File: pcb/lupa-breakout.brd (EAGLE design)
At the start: 40.3 x 40.6 mm, 16 parts

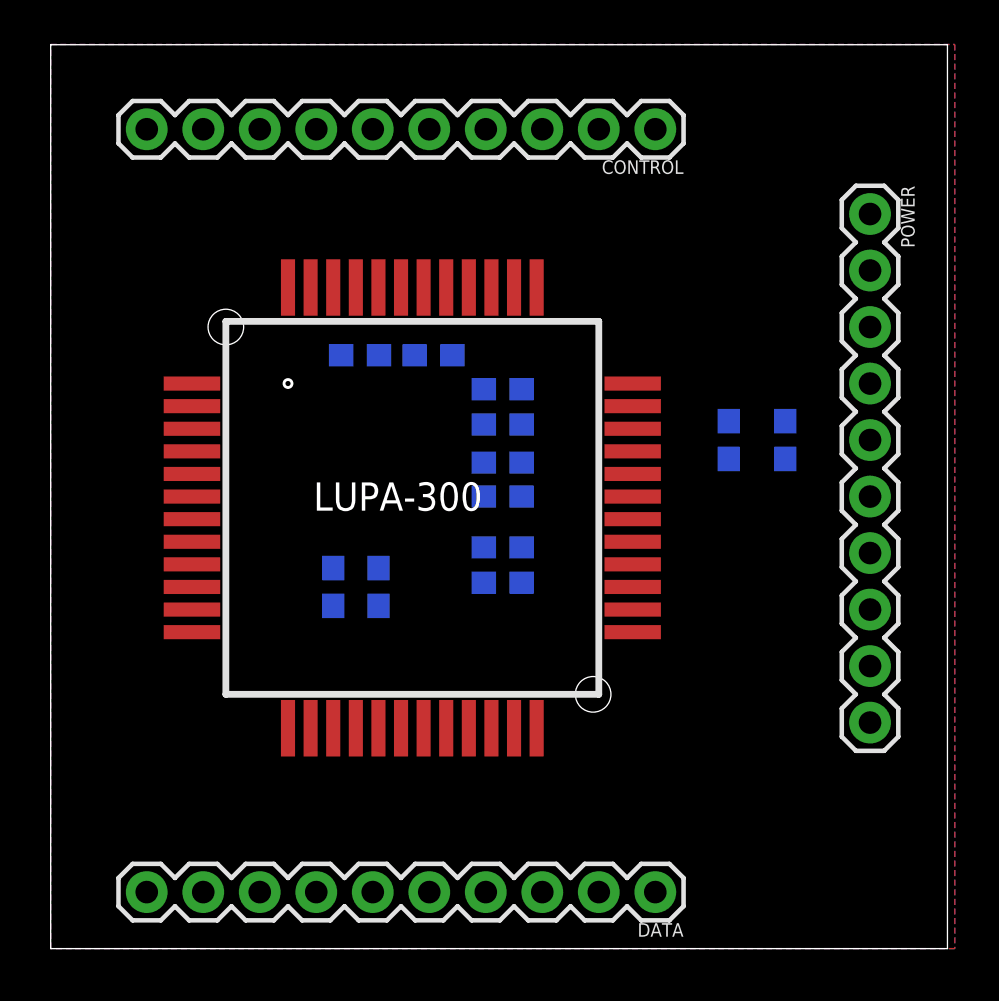
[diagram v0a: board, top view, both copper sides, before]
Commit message: more work on breakout
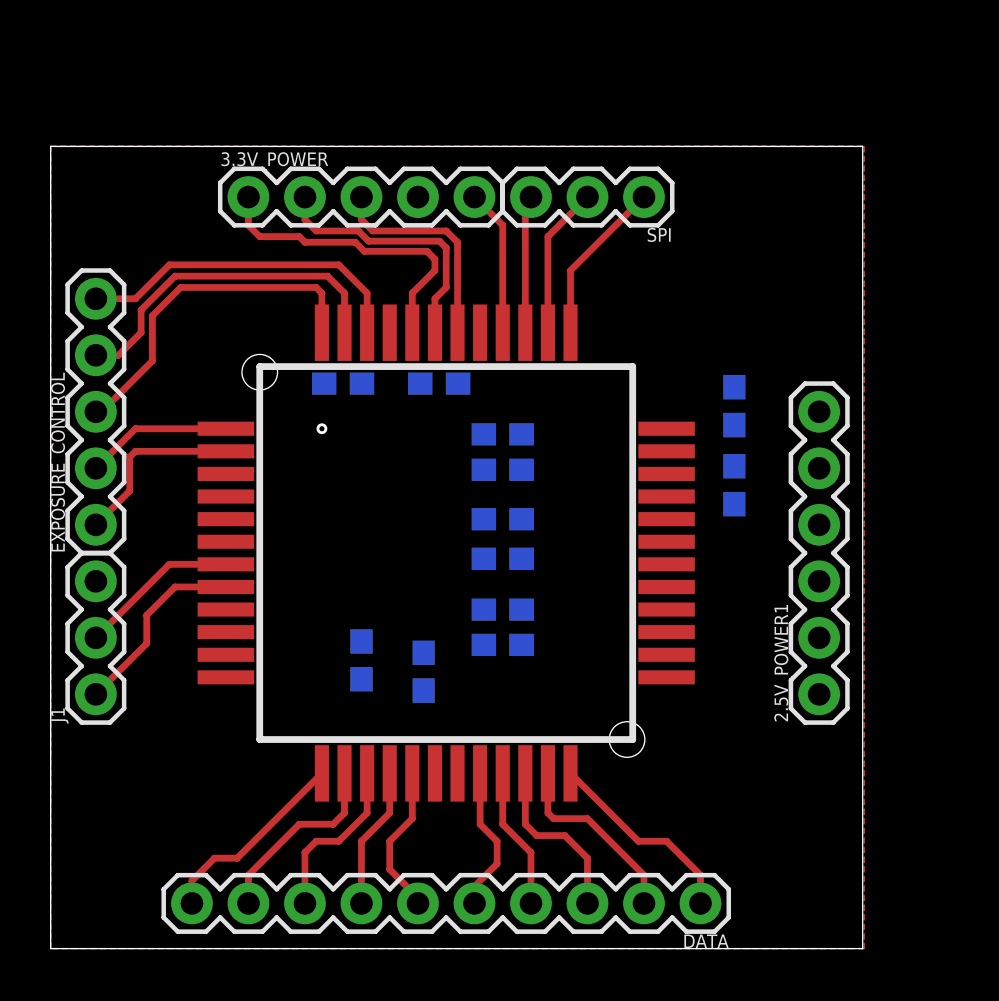
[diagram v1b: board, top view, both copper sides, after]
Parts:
- removed CONTROL, POWER: (no value), SparkFun-Connectors:1X10
- added 2.5V_POWER1: (no value), SparkFun-Connectors:1X06
- added 3.3V_POWER, EXPOSURE_CONTROL: (no value), SparkFun-Connectors:1X05
- added J1, SPI: 455-1750-1-ND, SparkFun-Connectors:1X03
- moved C1 4.32 mm to (16.8, 12.4), turned to 270 degrees
- moved R1 3.54 mm to (14.0, 13.0), turned to 270 degrees
- moved C4 2.79 mm to (20.3, 13.7)
- moved R3 2.79 mm to (20.3, 17.5)
- moved R4 2.79 mm to (20.3, 15.2)
- moved C2 2.75 mm to (30.7, 24.4), turned to 90 degrees
- moved C3 2.54 mm to (20.3, 19.3)
- moved U$1 2.54 mm to (10.7, 10.7)
- moved DATA 2.09 mm to (29.2, 2.03)
- moved R2 2.05 mm to (30.7, 20.8)
- moved C5 2.03 mm to (20.3, 23.1)
- moved R5 2.03 mm to (20.3, 21.5)
- moved C6 1.48 mm to (13.1, 25.4)
- moved R6 1.30 mm to (17.5, 25.4)
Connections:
- net CLK: now also J1.1; no longer CONTROL.10
- net FRAME_VALID: now also EXPOSURE_CONTROL.4; no longer CONTROL.5
- net GND: now also 2.5V_POWER1.1, 3.3V_POWER.4, J1.3; no longer POWER.10
- net INT_TIME1: now also EXPOSURE_CONTROL.1; no longer CONTROL.8
- net INT_TIME2: now also EXPOSURE_CONTROL.2; no longer CONTROL.7
- net INT_TIME3: now also EXPOSURE_CONTROL.3; no longer CONTROL.6
- net LINE_VALID: now also EXPOSURE_CONTROL.5; no longer CONTROL.4
- net RESET: now also J1.2; no longer CONTROL.9
- net SPI_CLK: now also SPI.2; no longer CONTROL.2
- net SPI_DATA: now also SPI.3; no longer CONTROL.3
- net SPI_EN: now also SPI.1; no longer CONTROL.1
- net VADC: now also 2.5V_POWER1.4; no longer POWER.5
- net VDDA: now also 2.5V_POWER1.5; no longer POWER.7
- net VDDD: now also 2.5V_POWER1.3; no longer POWER.6
- net VDDO: now also 2.5V_POWER1.2; no longer POWER.4
- net VMEM_H: now also 3.3V_POWER.5; no longer POWER.8
- net VPIX: now also 2.5V_POWER1.6; no longer POWER.3
- net VRESET_1: now also 3.3V_POWER.3; no longer POWER.9
- net VRESET_2: now also 3.3V_POWER.2; no longer POWER.2
- net VRESET_3: now also 3.3V_POWER.1; no longer POWER.1
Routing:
- net INT_TIME3: track 0.00 -> 15.5 mm
- net FRAME_VALID: track 0.00 -> 15.3 mm
- net LINE_VALID: track 0.00 -> 15.1 mm
- net VRESET_3: track 0.00 -> 14.0 mm
- net VRESET_2: track 0.00 -> 11.9 mm
- net VRESET_1: track 0.00 -> 9.82 mm
- net D9: track 0.00 -> 9.01 mm
- net D0: track 0.00 -> 8.86 mm
- net CLK: track 0.00 -> 8.58 mm
- net D8: track 0.00 -> 8.52 mm
- net D1: track 0.00 -> 8.52 mm
- net INT_TIME1: track 0.00 -> 8.10 mm
- net D7: track 0.00 -> 7.74 mm
- net D2: track 0.00 -> 7.59 mm
- net SPI_EN: track 0.00 -> 7.46 mm
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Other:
- board size 40.3 x 40.6 mm -> 36.5 x 36.1 mm
